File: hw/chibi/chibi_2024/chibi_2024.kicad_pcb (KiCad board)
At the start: 2 copper layers, 101.6 x 78.2 mm, 114 parts, among them P1 VIN, P2 VIN, P3 GND, P4 CONN_02X05, P5 SWD, P6 GND, Q1 AO3415A, Q10 Q_NPN_CBE, Q11 Q_NPN_CBE, Q2 AO3415A, Q3 AO3415A, Q4 AO3415A, Q5 AO3415A, Q6 AO3415A, Q7 AO3415A, Q8 AO3415A, Q9 Q_PNP_CBE, SW1 USER, SW2 RESET, U1 LD1117S33CTR, U2 SP3485CN, U3 STM32F030F4Px, U4 LM358, U5 74HC595_mine, U6 LM393, U7 74HC595_mine, U8 MBI5026, U9 MBI5026, Y1 8MHz

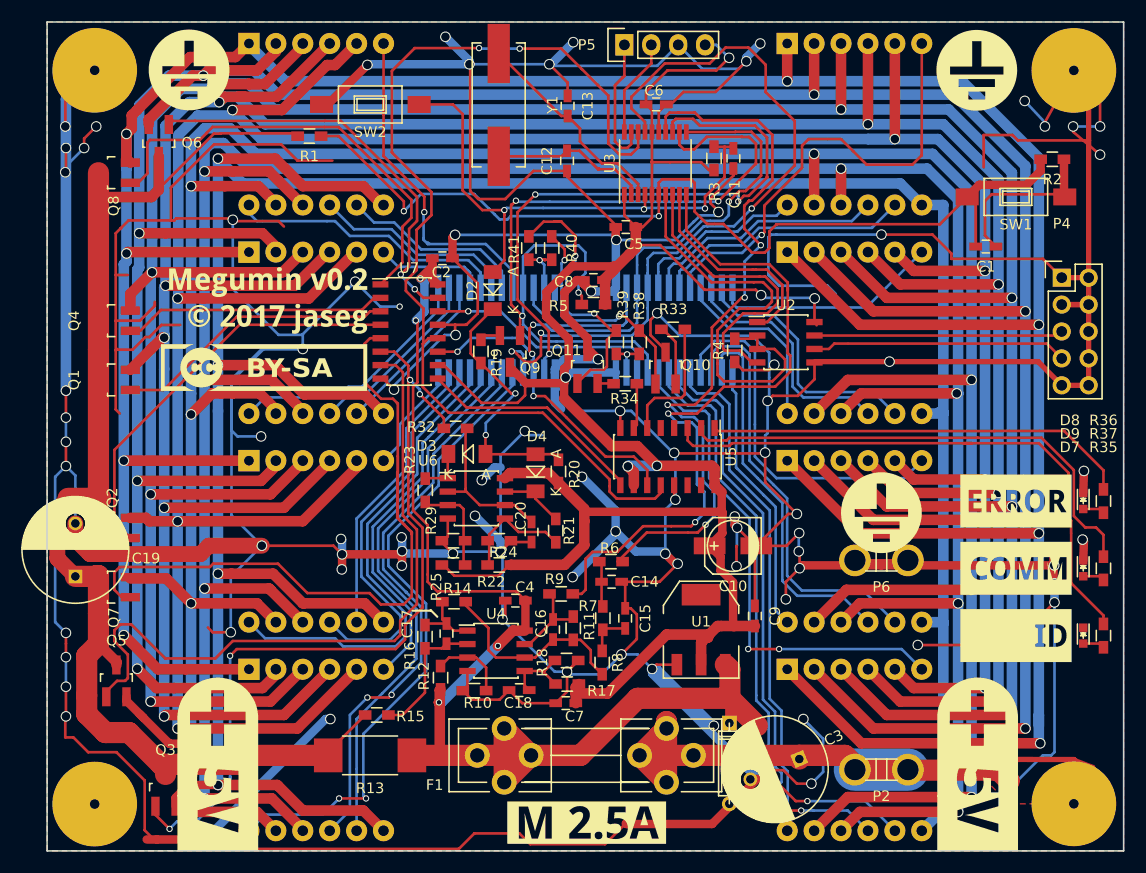
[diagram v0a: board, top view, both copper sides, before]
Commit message: foo
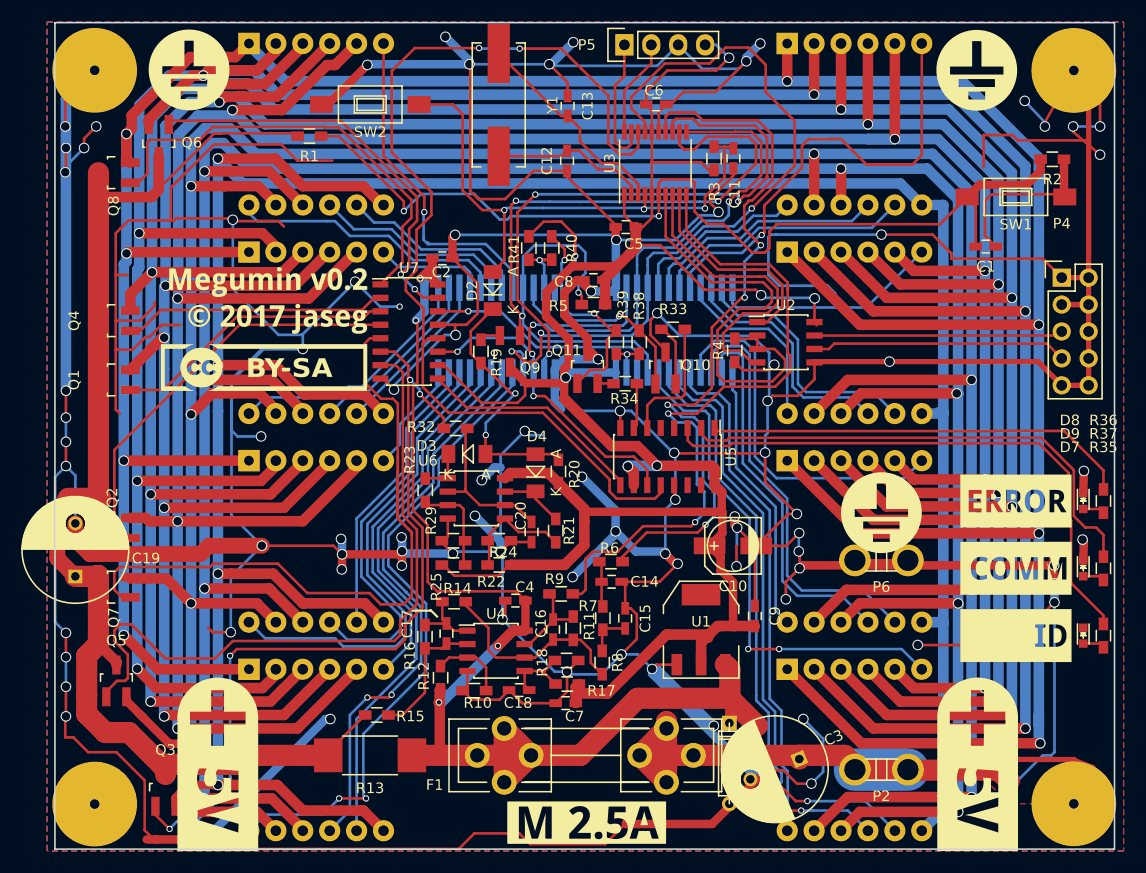
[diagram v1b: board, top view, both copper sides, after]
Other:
- board size 101.6 x 78.2 mm -> 100 x 78 mm
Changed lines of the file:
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@@
     (links 308)
     (no_connects 0)
-    (area 45.401999 39.515396 153.957624 125.872685)
+    (area 48.184999 43.612999 149.935001 121.995001)
     (thickness 1.6)
     (drawings 6)
@@
       (net 99 /mux_mod_left/VDD))
   )
+  (gr_line (start 149 121.75) (end 149 43.75) (angle 90) (layer Edge.Cuts) (width 0.15))
+  (gr_line (start 149 43.75) (end 49 43.75) (angle 90) (layer Edge.Cuts) (width 0.15))
+  (gr_line (start 49 121.75) (end 149 121.75) (angle 90) (layer Edge.Cuts) (width 0.15))
+  (gr_line (start 49 43.75) (end 49 121.75) (angle 90) (layer Edge.Cuts) (width 0.15))
   (gr_line (start 84.5 99.25) (end 82.75 99.25) (angle 90) (layer F.SilkS) (width 0.2))
-  (gr_line (start 48.26 121.92) (end 48.26 43.688) (angle 90) (layer Edge.Cuts) (width 0.15))
-  (gr_line (start 149.86 121.92) (end 48.26 121.92) (angle 90) (layer Edge.Cuts) (width 0.15))
-  (gr_line (start 149.86 43.688) (end 149.86 121.92) (angle 90) (layer Edge.Cuts) (width 0.15))
-  (gr_line (start 48.26 43.688) (end 149.86 43.688) (angle 90) (layer Edge.Cuts) (width 0.15))
   (gr_line (start 84.455 99.187) (end 85.09 99.822) (angle 90) (layer F.SilkS) (width 0.2))
   (segment (start 67.299998 49.549998) (end 68.25 49.549998) (width 1) (layer F.Cu) (net 0))
@@
   (segment (start 57.9115 73.4235) (end 59.0545 72.2805) (width 0.254) (layer F.Cu) (net 3))
   (segment (start 59.0545 72.2805) (end 60.8325 72.2805) (width 0.254) (layer F.Cu) (net 3))
-  (segment (start 52.75 48.25) (end 49.974 51.026) (width 0.254) (layer F.Cu) (net 3))
-  (segment (start 49.974 51.026) (end 49.974 53.548) (width 0.254) (layer F.Cu) (net 3))
+  (segment (start 52.75 48.25) (end 49.974 51.026) (width 0.254) (layer F.Cu) (net 3) (status 30))
+  (segment (start 49.974 51.026) (end 49.974 53.548) (width 0.254) (layer F.Cu) (net 3) (status 10))
   (via (at 52.895 53.548) (size 1) (drill 0.8) (layers F.Cu B.Cu) (net 3))
   (segment (start 51.752 54.691) (end 52.895 53.548) (width 0.254) (layer F.Cu) (net 3))
@@
   (segment (start 147.637 53.548) (end 145.097 53.548) (width 0.254) (layer B.Cu) (net 3))
   (via (at 147.637 53.548) (size 1) (drill 0.8) (layers F.Cu B.Cu) (net 3))
-  (segment (start 52.75 48.25) (end 55.453 45.547) (width 0.254) (layer F.Cu) (net 3))
+  (segment (start 52.75 48.25) (end 55.453 45.547) (width 0.254) (layer F.Cu) (net 3) (status 30))
   (segment (start 49.9745 111.206) (end 50.736 111.206) (width 0.254) (layer F.Cu) (net 3))
   (segment (start 58.61 120.985) (end 58.61 120.8405) (width 0.254) (layer F.Cu) (net 3))
@@
   (segment (start 52.133 112.603) (end 54.8 112.603) (width 0.254) (layer F.Cu) (net 3))
   (segment (start 50.736 111.206) (end 52.133 112.603) (width 0.254) (layer F.Cu) (net 3))
-  (segment (start 50.038 50.962) (end 50.038 78.486) (width 1) (layer B.Cu) (net 3))
+  (segment (start 50.038 50.962) (end 50.038 78.486) (width 1) (layer B.Cu) (net 3) (status 10))
   (via (at 50.038 85.598) (size 1) (drill 0.8) (layers F.Cu B.Cu) (net 3))
   (segment (start 50.038 83.312) (end 50.038 85.598) (width 0.254) (layer F.Cu) (net 3))
@@
   (segment (start 50.038 78.486) (end 50.038 81.026) (width 0.254) (layer F.Cu) (net 3))
   (via (at 50.038 78.486) (size 1) (drill 0.8) (layers F.Cu B.Cu) (net 3))
-  (segment (start 50.038 50.962) (end 52.75 48.25) (width 1) (layer B.Cu) (net 3))
+  (segment (start 50.038 50.962) (end 52.75 48.25) (width 1) (layer B.Cu) (net 3) (status 30))
   (segment (start 50.038 85.598) (end 50.927 86.487) (width 0.25) (layer B.Cu) (net 3))
   (segment (start 50.927 86.487) (end 50.927 91.012) (width 0.25) (layer B.Cu) (net 3))
